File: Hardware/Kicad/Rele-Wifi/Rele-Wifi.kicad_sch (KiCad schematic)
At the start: 20 parts, among them U1 817C, U2 817C

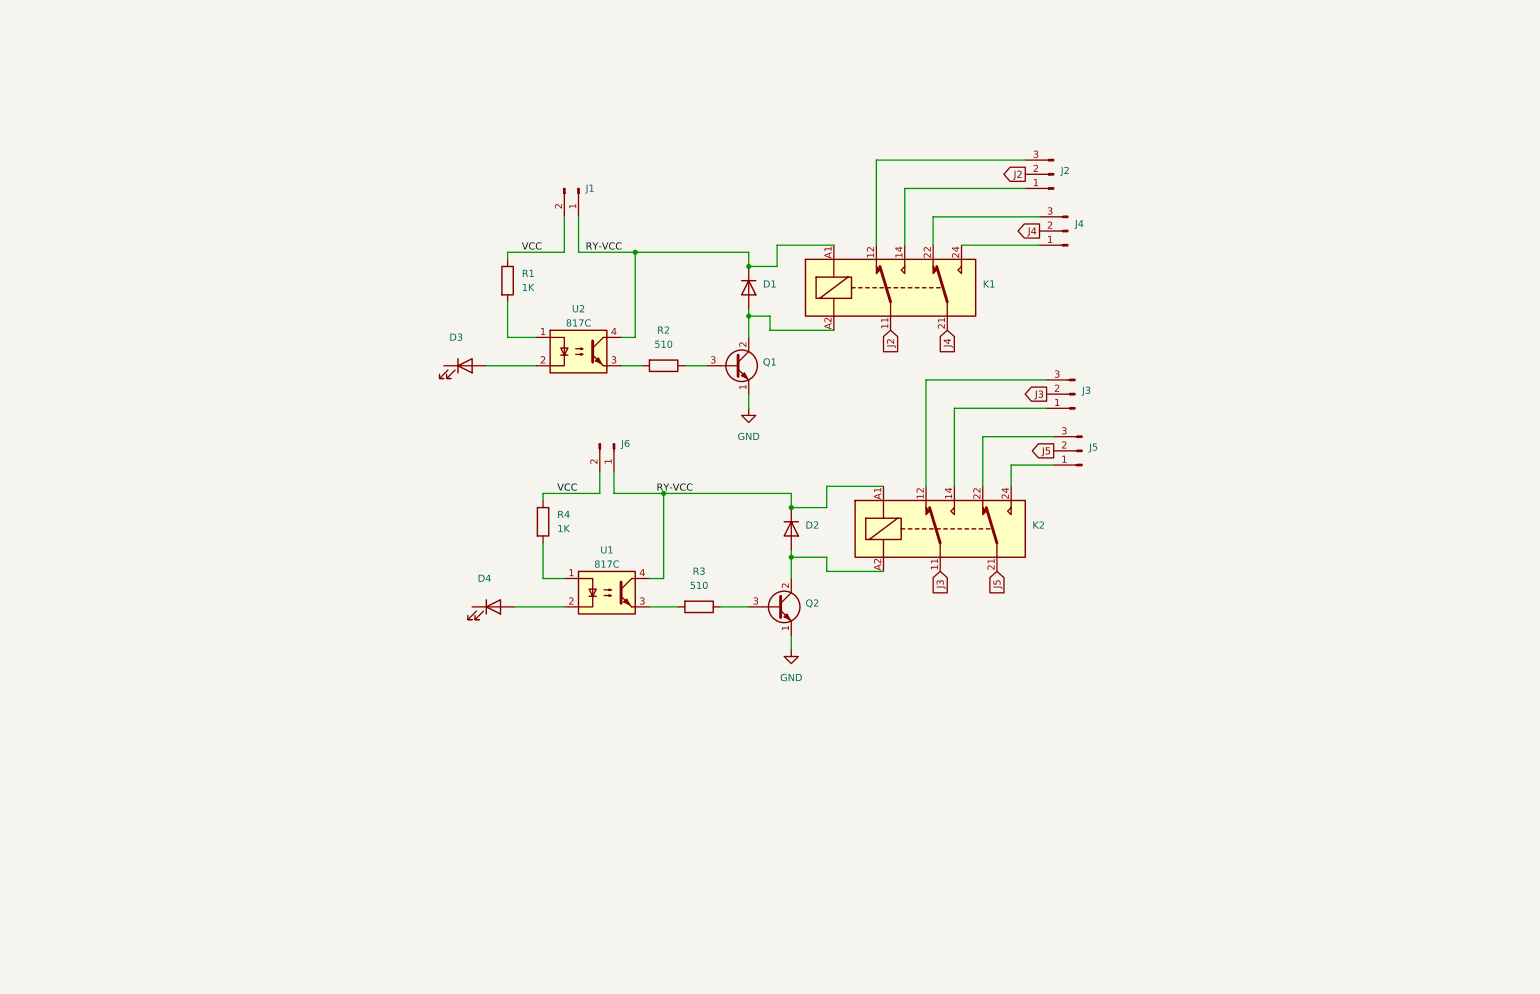
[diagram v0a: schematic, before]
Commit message: Terminamos el esquematico
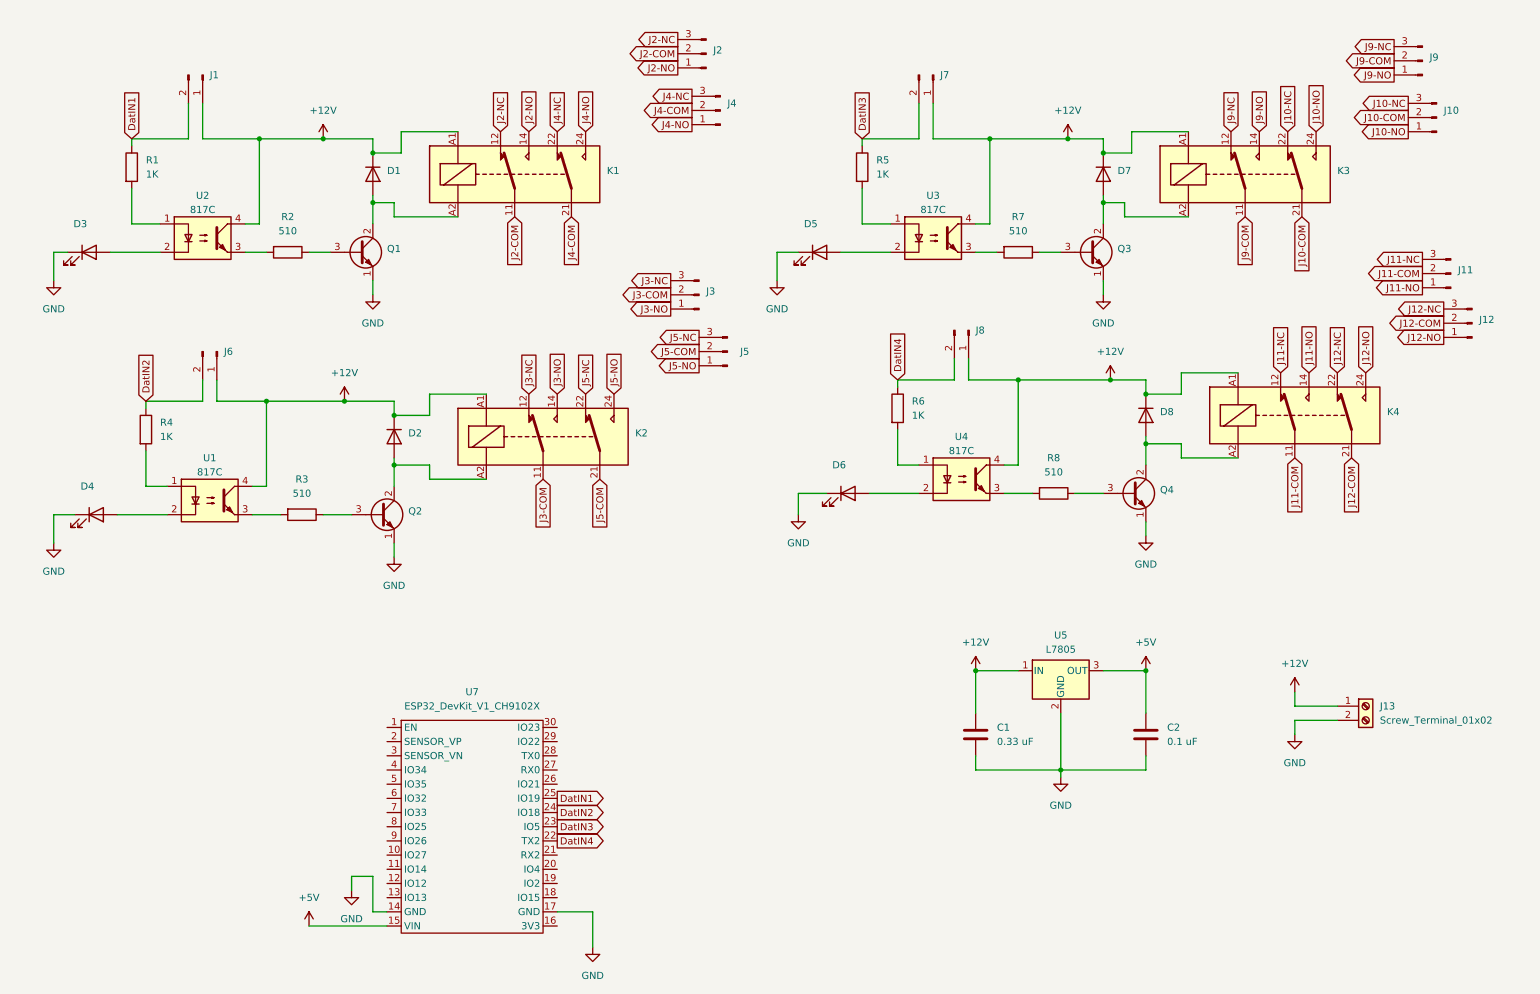
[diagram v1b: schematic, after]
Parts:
- added C1: 0.33 uF, Capacitor_SMD:C_0805_2012Metric, symbol Device:C
- added C2: 0.1 uF, Capacitor_SMD:C_0805_2012Metric, symbol Device:C
- added D5, D6: ~, EESTN5:Led_0805, symbol Device:LED
- added D7, D8: ~, Diode_SMD:D_0805_2012Metric, symbol Device:D
- added J10, J11, J12, J9: ~, TerminalBlock:TerminalBlock_Xinya_XY308-2.54-3P_1x03_P2.54mm_Horizontal, symbol Connector:Conn_01x03_Pin
- added J13: Screw_Terminal_01x02, TerminalBlock:TerminalBlock_bornier-2_P5.08mm, symbol Connector:Screw_Terminal_01x02
- added J7, J8: ~, EESTN5:Jumper, symbol Connector:Conn_01x02_Pin
- added K3, K4: ~, Relay_THT:Relay_DPDT_Finder_30.22, symbol Relay:HK19F-DCxxV-SHC
- added Q3, Q4: ~, Package_TO_SOT_SMD:SOT-23, symbol Transistor_BJT:BF457
- added R5, R6: 1K, Resistor_SMD:R_0805_2012Metric_Pad1.20x1.40mm_HandSolder, symbol Device:R
- added R7, R8: 510, Resistor_SMD:R_0805_2012Metric_Pad1.20x1.40mm_HandSolder, symbol Device:R
- added U3, U4: 817C, Package_DIP:DIP-4_W7.62mm, symbol Isolator:EL817
- added U5: L7805, Package_TO_SOT_SMD:TO-263-3_TabPin2, symbol Regulator_Linear:L7805
- added U7: ESP32_DevKit_V1_CH9102X, EESTN5:ESP32-WROOM-32.30pines, symbol EESTN5:ESP32_DevKit_V1_CH9102X
- J2, J3, J4, J5: footprint TerminalBlock:TerminalBlock_MaiXu_MX126-5.0-03P_1x03_P5.00mm -> TerminalBlock:TerminalBlock_Xinya_XY308-2.54-3P_1x03_P2.54mm_Horizontal
- Q1, Q2: footprint Package_TO_SOT_THT:TO-126-3_Vertical -> Package_TO_SOT_SMD:SOT-23
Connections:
- net GND: now also D3.1 (K), D4.1 (K), C1.2, C2.2, D5.1 (K), D6.1 (K), J13.2 (Pin_2), Q3.1 (E), Q4.1 (E), U5.2 (GND), U7.14 (GND), U7.17 (GND)
- net J3-NO: now reaches J3.1 (Pin_1), K2.14
- net J3-NC: now reaches J3.3 (Pin_3), K2.12
- net J2-NC: now reaches J2.3 (Pin_3), K1.12
- net J2-NO: now reaches J2.1 (Pin_1), K1.14
- net J4-NC: now reaches J4.3 (Pin_3), K1.22
- net J4-NO: now reaches J4.1 (Pin_1), K1.24
- net J5-NC: now reaches J5.3 (Pin_3), K2.22
- net J5-NO: now reaches J5.1 (Pin_1), K2.24
- net J2 renamed J2-COM
- net J3 renamed J3-COM
- net J4 renamed J4-COM
- net J5 renamed J5-COM
- net RY-VCC renamed +12V
- net +12V: now also C1.1, D7.1 (K), D8.1 (K), J13.1 (Pin_1), J7.1 (Pin_1), J8.1 (Pin_1), K3.A1, K4.A1, U3.4, U4.4, U5.1 (IN)
- net VCC renamed DatIN1
- net DatIN1: now also U7.25 (IO19); no longer J6.2 (Pin_2), R4.1
- new net: D7.2 (A), K3.A2, Q3.2 (C)
- new net: Q3.3 (B), R7.1
- new net: Q4.3 (B), R8.1
- new net: R8.2, U4.3
- new net: D8.2 (A), K4.A2, Q4.2 (C)
- new net: R5.2, U3.1
- new net: R7.2, U3.3
- new net: D5.2 (A), U3.2
- new net: D6.2 (A), U4.2
- new net: R6.2, U4.1
- new net +5V: C2.1, U5.3 (OUT), U7.15 (VIN)
- new net DatIN2: J6.2 (Pin_2), R4.1, U7.24 (IO18)
- new net DatIN3: J7.2 (Pin_2), R5.1, U7.23 (IO5)
- new net DatIN4: J8.2 (Pin_2), R6.1, U7.22 (TX2)
- new net J10-COM: J10.2 (Pin_2), K3.21
- new net J10-NC: J10.3 (Pin_3), K3.22
- new net J10-NO: J10.1 (Pin_1), K3.24
- new net J11-COM: J11.2 (Pin_2), K4.11
- new net J11-NC: J11.3 (Pin_3), K4.12
- new net J11-NO: J11.1 (Pin_1), K4.14
- new net J12-COM: J12.2 (Pin_2), K4.21
- new net J12-NC: J12.3 (Pin_3), K4.22
- new net J12-NO: J12.1 (Pin_1), K4.24
- new net J9-COM: J9.2 (Pin_2), K3.11
- new net J9-NC: J9.3 (Pin_3), K3.12
- new net J9-NO: J9.1 (Pin_1), K3.14
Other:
- moved on the sheet: D1, D2, D3, D4, J1, J2, J3, J4, J5, J6, K1, K2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

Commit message: Terminamos el pcb
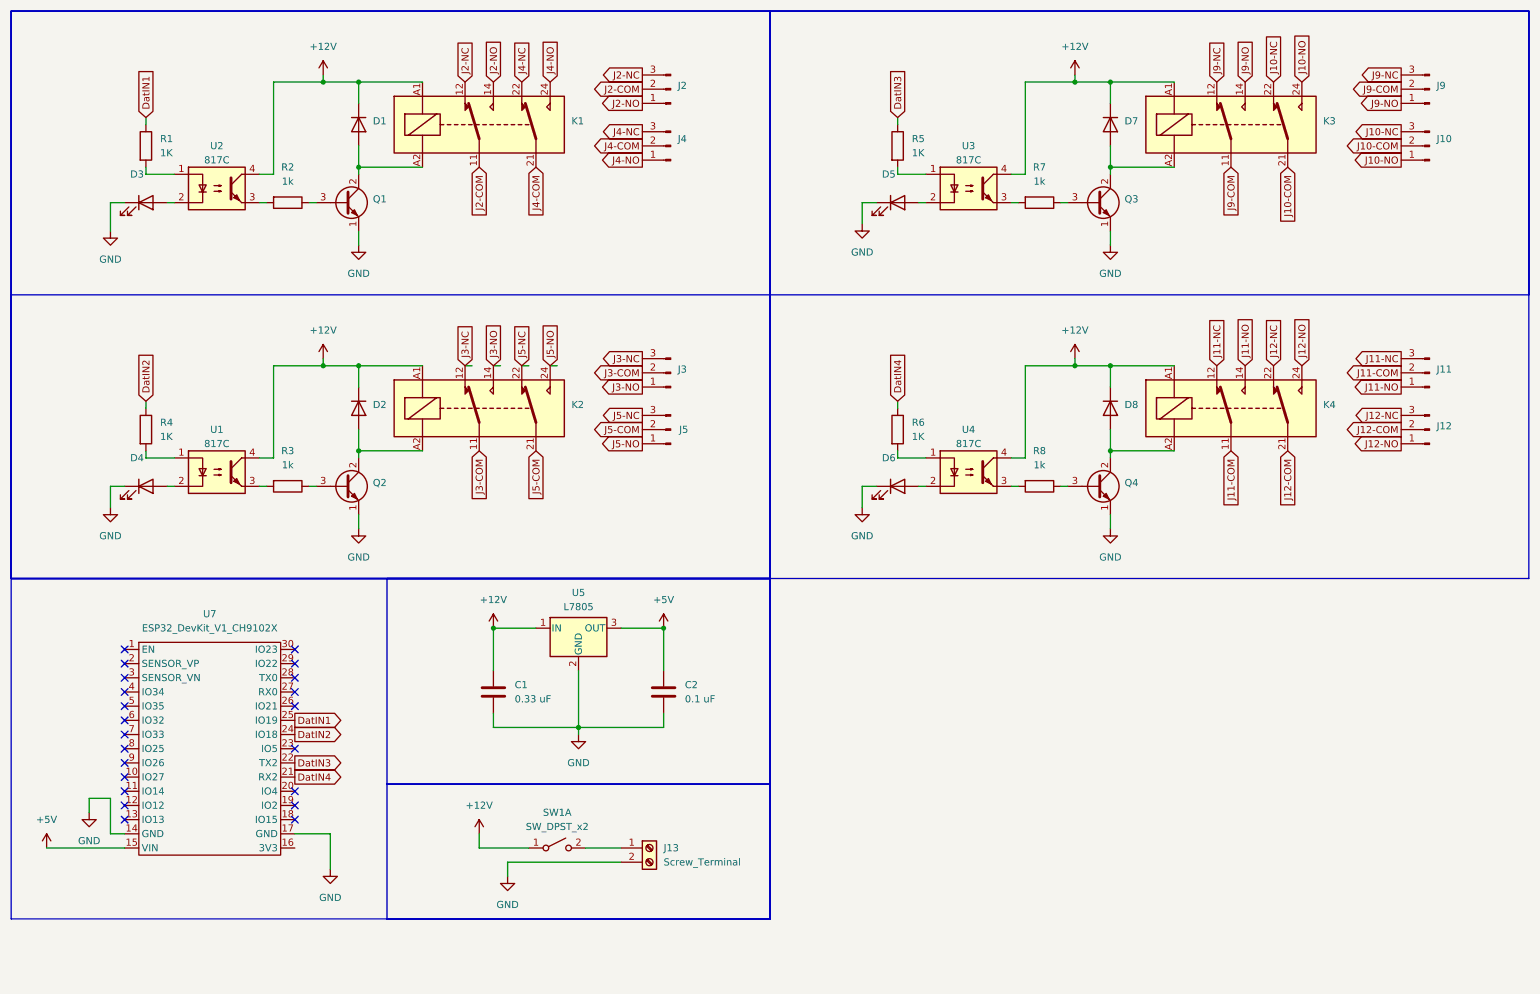
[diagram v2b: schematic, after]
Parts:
- removed J1, J6, J7, J8: ~, EESTN5:Jumper, symbol Connector:Conn_01x02_Pin
- added SW1: SW_DPST_x2, Button_Switch_THT:SW_PUSH_1P1T_6x3.5mm_H4.3_APEM_MJTP1243, symbol Switch:SW_DPST_x2
- J13: value Screw_Terminal_01x02 -> Screw_Terminal
- R2, R3, R7, R8: value 510 -> 1k
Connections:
- net +12V: now also SW1.1 (A); no longer J13.1 (Pin_1)
- net DatIN3: now also U7.22 (TX2); no longer U7.23 (IO5)
- net DatIN4: now also U7.21 (RX2); no longer U7.22 (TX2)
- new net: J13.1 (Pin_1), SW1.2 (B)
- no-connect marks 0 -> 22
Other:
- moved on the sheet: C1, C2, D1, D2, D3, D4, D5, D6, D7, D8, J10, J11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

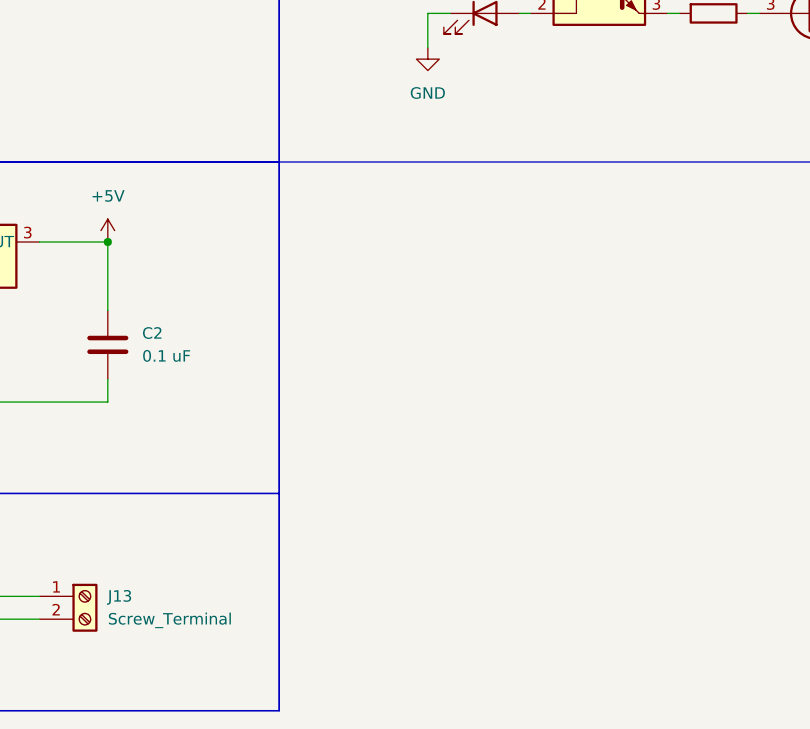
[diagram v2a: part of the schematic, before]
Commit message: Para el Chequeo de Legui
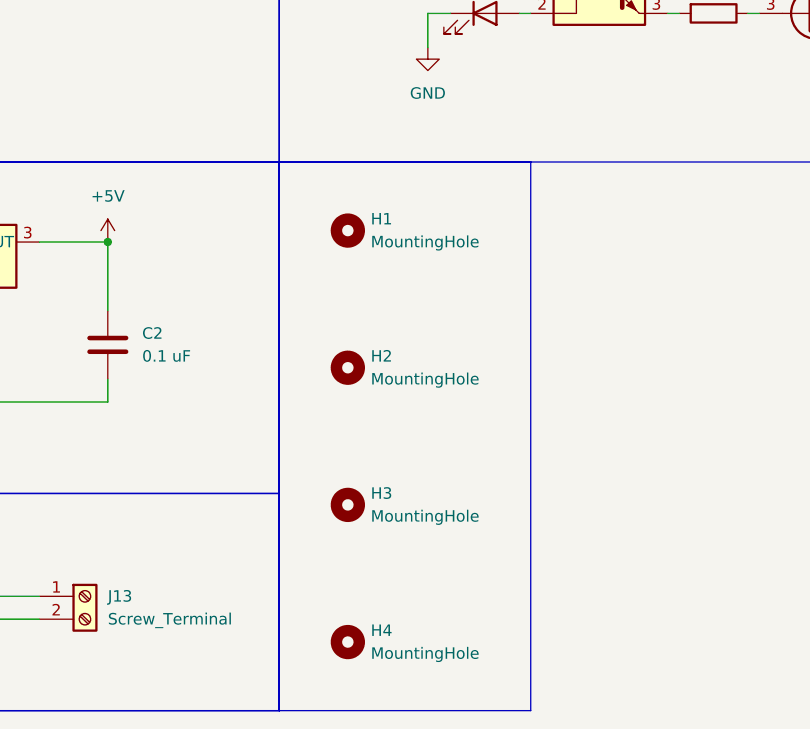
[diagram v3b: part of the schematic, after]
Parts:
- added H1, H2, H3, H4: MountingHole, MountingHole:MountingHole_3.2mm_M3, symbol Mechanical:MountingHole
- J13: footprint TerminalBlock:TerminalBlock_bornier-2_P5.08mm -> TerminalBlock:TerminalBlock_MaiXu_MX126-5.0-02P_1x02_P5.00mm
